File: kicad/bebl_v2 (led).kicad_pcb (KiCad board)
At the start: 2 copper layers, 60 x 14 mm, 14 parts, among them P10 LED_DRL, P13 LED_CHG, P9 LED_DRV

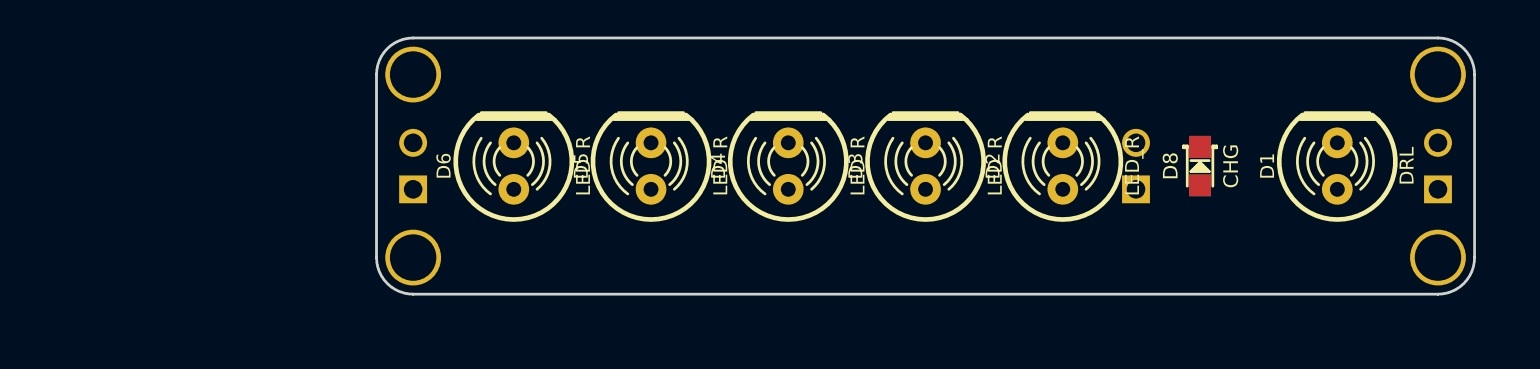
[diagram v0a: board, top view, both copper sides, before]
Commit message: bebl_v2 3d of housing, work in progress
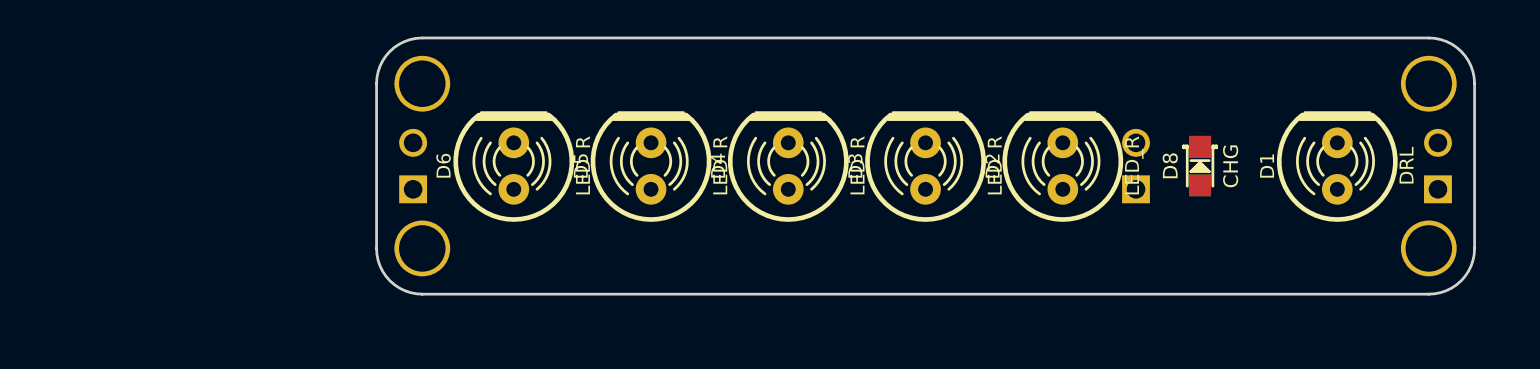
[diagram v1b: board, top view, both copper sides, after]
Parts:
- moved SC10 0.71 mm to (55.0, 74.5)
- moved SC11 0.71 mm to (110.0, 74.5)
- moved SC12 0.71 mm to (110.0, 65.5)
- moved SC9 0.71 mm to (55.0, 65.5)
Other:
- outline, holes or cut-outs redrawn
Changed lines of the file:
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@@
-(kicad_pcb (version 4) (host pcbnew "(2014-09-25 BZR 5147)-product")
+(kicad_pcb (version 4) (host pcbnew "(2014-jul-16 BZR unknown)-product")
   (general
     (links 10)
     (no_connects 10)
-    (area 48.6707 62.924999 112.7733 77.075001)
+    (area 48.6707 62.924999 112.575001 77.075001)
     (thickness 1.6)
     (drawings 8)
@@
   )
   (module bebl_v2_pretty:screw_3mm (layer F.Cu)
-    (at 110.5 65)
+    (at 110 65.5)
     (descr "vite 2,5mm")
     (fp_text reference SC12 (at 0 1.0795) (layer F.SilkS) hide
@@
   )
   (module bebl_v2_pretty:screw_3mm (layer F.Cu)
-    (at 110.5 75)
+    (at 110 74.5)
     (descr "vite 2,5mm")
     (fp_text reference SC11 (at 0 1.0795) (layer F.SilkS) hide
@@
   )
   (module bebl_v2_pretty:screw_3mm (layer F.Cu)
-    (at 54.5 75)
+    (at 55 74.5)
     (descr "vite 2,5mm")
     (fp_text reference SC10 (at 0 1.0795) (layer F.SilkS) hide
@@
   )
   (module bebl_v2_pretty:screw_3mm (layer F.Cu)
-    (at 54.5 65)
+    (at 55 65.5)
     (descr "vite 2,5mm")
     (fp_text reference SC9 (at 0 1.0795) (layer F.SilkS) hide
@@
     )
   )
-  (gr_line (start 110.5 63) (end 54.5 63) (angle 90) (layer Edge.Cuts) (width 0.15))
-  (gr_line (start 112.5 75) (end 112.5 65) (angle 90) (layer Edge.Cuts) (width 0.15))
-  (gr_line (start 54.5 77) (end 110.5 77) (angle 90) (layer Edge.Cuts) (width 0.15))
-  (gr_line (start 52.5 65) (end 52.5 75) (angle 90) (layer Edge.Cuts) (width 0.15))
-  (gr_arc (start 54.5 65) (end 52.5 65) (angle 90) (layer Edge.Cuts) (width 0.15))
-  (gr_arc (start 54.5 75) (end 54.5 77) (angle 90) (layer Edge.Cuts) (width 0.15))
-  (gr_arc (start 110.5 75) (end 112.5 75) (angle 90) (layer Edge.Cuts) (width 0.15))
-  (gr_arc (start 110.5 65) (end 110.5 63) (angle 90) (layer Edge.Cuts) (width 0.15))
+  (gr_line (start 112.5 74.5) (end 112.5 65.5) (angle 90) (layer Edge.Cuts) (width 0.15))
+  (gr_line (start 55 77) (end 110 77) (angle 90) (layer Edge.Cuts) (width 0.15))
+  (gr_line (start 52.5 65.5) (end 52.5 74.5) (angle 90) (layer Edge.Cuts) (width 0.15))
+  (gr_line (start 110 63) (end 55 63) (angle 90) (layer Edge.Cuts) (width 0.15))
+  (gr_arc (start 110 65.5) (end 110 63) (angle 90) (layer Edge.Cuts) (width 0.15))
+  (gr_arc (start 110 74.5) (end 112.5 74.5) (angle 90) (layer Edge.Cuts) (width 0.15))
+  (gr_arc (start 55 74.5) (end 55 77) (angle 90) (layer Edge.Cuts) (width 0.15))
+  (gr_arc (start 55 65.5) (end 52.5 65.5) (angle 90) (layer Edge.Cuts) (width 0.15))
 )

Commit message: working on case for bebl_v2
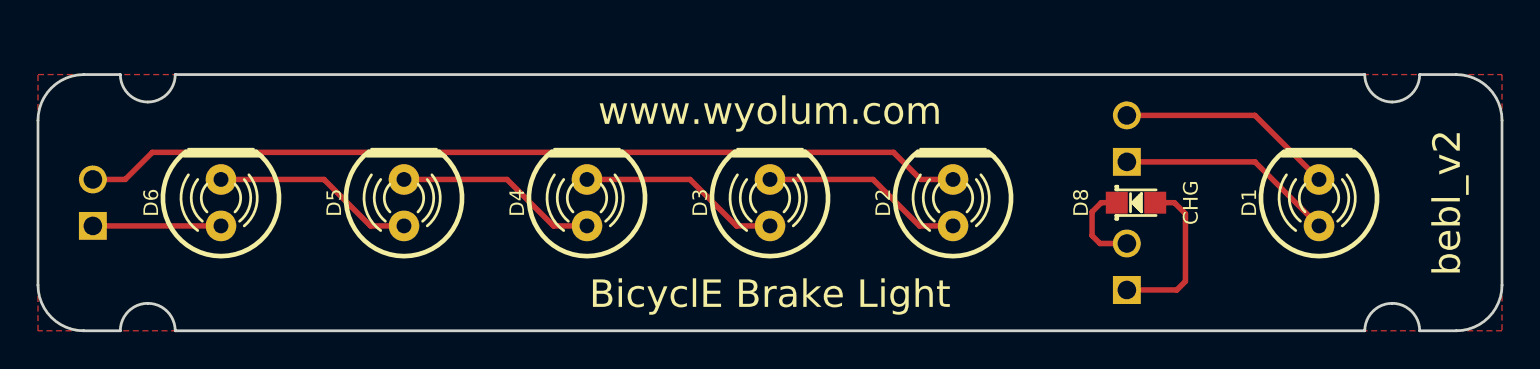
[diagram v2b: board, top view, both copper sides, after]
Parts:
- removed SC10, SC11, SC12, SC9: SCREW, bebl_v2_pretty:screw_3mm
- moved P9 17.6 mm to (37.0, 72.0)
- moved P10 17.1 mm to (93.5, 68.5)
- moved D6 16.1 mm to (44.0, 72.0)
- moved D5 13.6 mm to (54.0, 72.0)
- moved D4 11.2 mm to (64.0, 72.0)
- moved D3 8.73 mm to (74.0, 72.0)
- moved D2 6.32 mm to (84.0, 72.0)
- moved P13 5.52 mm to (93.5, 75.5)
- moved D8 4.03 mm to (94.0, 72.0), turned to 180 degrees
- moved D1 2.24 mm to (104.0, 72.0)
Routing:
- net /CATH: track 0.00 -> 48.2 mm
- net /D1K: track 0.00 -> 11.9 mm
- net /D1A: track 0.00 -> 11.9 mm
- net Net-(D5-Pad1): track 0.00 -> 11.1 mm
- net Net-(D4-Pad1): track 0.00 -> 11.1 mm
- net Net-(D3-Pad1): track 0.00 -> 11.1 mm
- net Net-(D2-Pad1): track 0.00 -> 11.1 mm
- net Net-(D8-Pad1): track 0.00 -> 8.99 mm
- net /ANOD: track 0.00 -> 7.00 mm
- net Net-(D8-Pad2): track 0.00 -> 4.94 mm
- added copper zone on F.Cu, net /D1K
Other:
- board size 60 x 14 mm -> 80 x 14 mm
- net class 0.2mm added: clearance 0.2, trace_width 0.2, via_dia 0.889, via_drill 0.635
- net class Default: clearance 0.254 -> 0.25; trace_width 0.254 -> 0.3
- rule trace_clearance: 0.254 -> 0.25
- rule trace_min: 0.254 -> 0.2
- board text added: "BicyclE Brake Light"
- board text added: "bebl_v2"
- board text added: "www.wyolum.com"
